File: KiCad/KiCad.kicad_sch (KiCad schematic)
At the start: 21 parts, among them J2 Conn_01x04, SW1 SW_Push, U1 ESP32-S3-WROOM-1

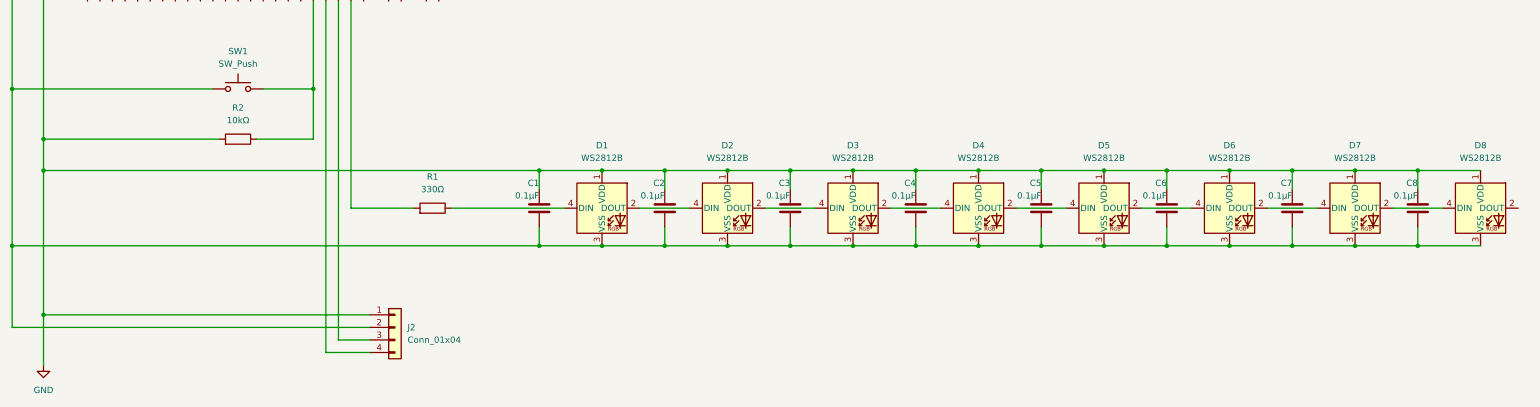
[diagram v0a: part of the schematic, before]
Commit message: CHG: minor changes to PCB
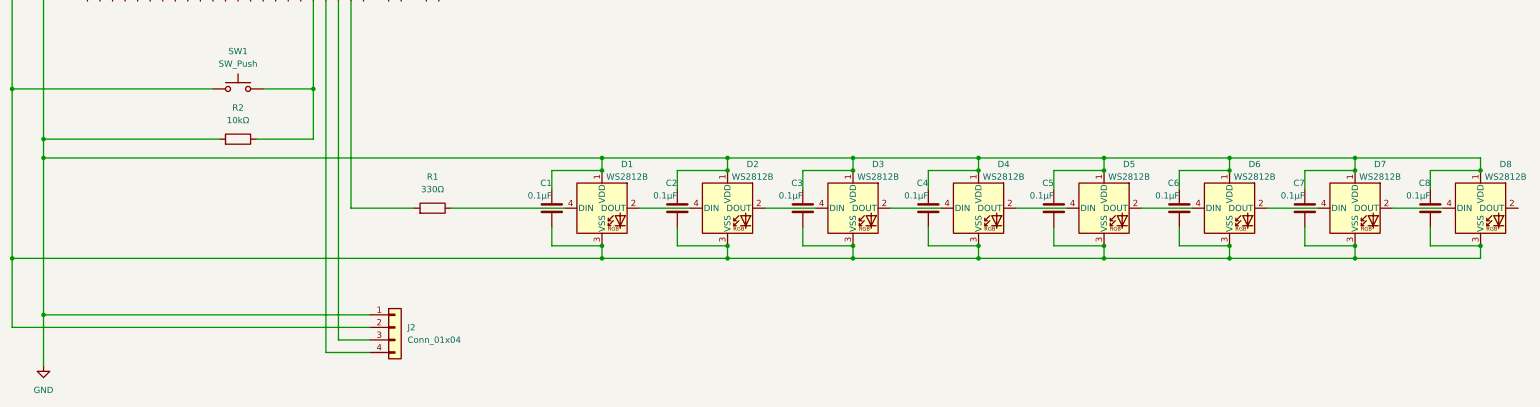
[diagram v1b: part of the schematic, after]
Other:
- moved on the sheet: C1, C2, C3, C4, C5, C6, C7, C8
